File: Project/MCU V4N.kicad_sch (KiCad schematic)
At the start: 10 parts, among them U59 STM32F072CBT6

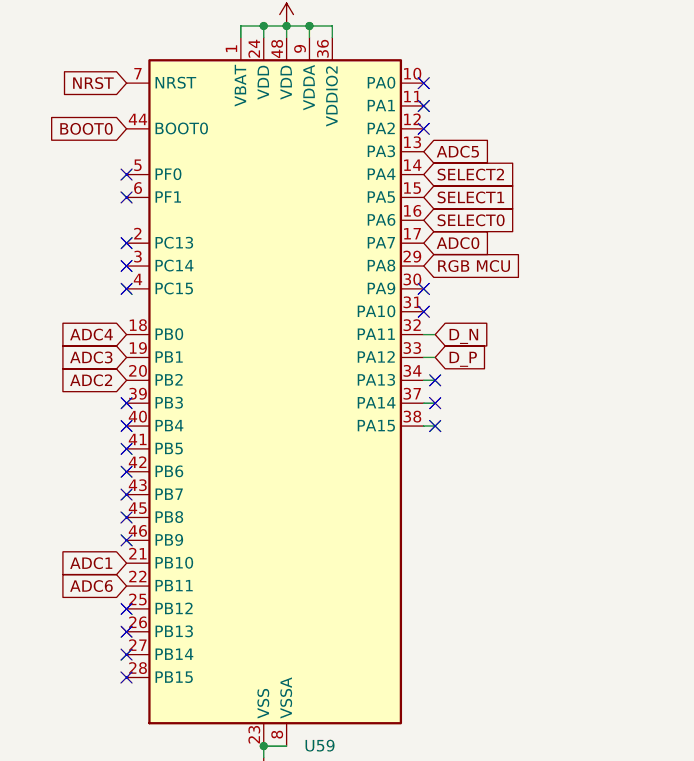
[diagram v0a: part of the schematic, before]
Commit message: pin revision
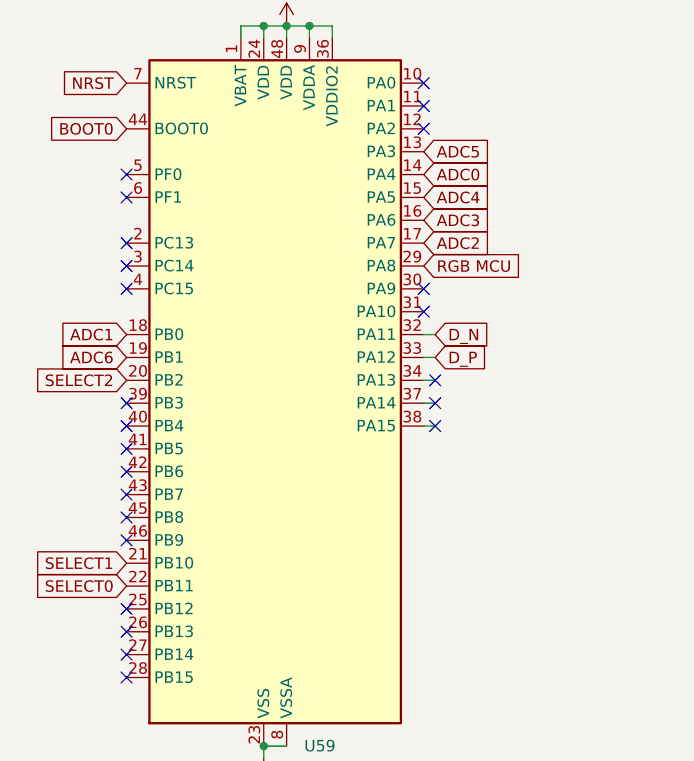
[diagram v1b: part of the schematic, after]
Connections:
- net ADC0: now also U59.14 (PA4); no longer U59.17 (PA7)
- net ADC1: now also U59.18 (PB0); no longer U59.21 (PB10)
- net ADC2: now also U59.17 (PA7); no longer U59.20 (PB2)
- net ADC3: now also U59.16 (PA6); no longer U59.19 (PB1)
- net ADC4: now also U59.15 (PA5); no longer U59.18 (PB0)
- net ADC6: now also U59.19 (PB1); no longer U59.22 (PB11)
- net SELECT0: now also U59.22 (PB11); no longer U59.16 (PA6)
- net SELECT1: now also U59.21 (PB10); no longer U59.15 (PA5)
- net SELECT2: now also U59.20 (PB2); no longer U59.14 (PA4)
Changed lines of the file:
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@@
   (no_connect (at 21.59 90.17))
   (no_connect (at 21.59 36.83))
+  (no_connect (at 54.61 24.13))
   (no_connect (at 21.59 34.29))
   (no_connect (at 21.59 44.45))
-  (no_connect (at 54.61 29.21))
   (no_connect (at 21.59 62.23))
   (no_connect (at 21.59 69.85))
   (no_connect (at 21.59 59.69))
+  (no_connect (at 54.61 29.21))
   (no_connect (at 54.61 46.99))
   (no_connect (at 21.59 67.31))
@@
   (no_connect (at 21.59 82.55))
   (no_connect (at 21.59 87.63))
+  (no_connect (at 54.61 26.67))
   (no_connect (at 55.88 59.69))
   (no_connect (at 21.59 46.99))
@@
   (no_connect (at 54.61 49.53))
   (no_connect (at 21.59 41.91))
-  (no_connect (at 54.61 24.13))
-  (no_connect (at 54.61 26.67))
   (wire (pts (xy 36.83 17.78) (xy 36.83 19.05))
     (stroke (width 0) (type default))
@@
     )
   )
-  (global_label "ADC3" (shape input) (at 21.59 54.61 180) (fields_autoplaced)
+  (global_label "ADC3" (shape input) (at 54.61 39.37 0) (fields_autoplaced)
+    (effects (font (size 1.27 1.27)) (justify left))
+    (property "Intersheetrefs" "${INTERSHEET_REFS}" (at 61.6997 39.37 0)
+      (effects (font (size 1.27 1.27)) (justify left) hide)
+    )
+  )
+  (global_label "ADC5" (shape input) (at 54.61 31.75 0) (fields_autoplaced)
+    (effects (font (size 1.27 1.27)) (justify left))
+    (property "Intersheetrefs" "${INTERSHEET_REFS}" (at 61.6997 31.75 0)
+      (effects (font (size 1.27 1.27)) (justify left) hide)
+    )
+  )
+  (global_label "ADC0" (shape input) (at 54.61 34.29 0) (fields_autoplaced)
+    (effects (font (size 1.27 1.27)) (justify left))
+    (property "Intersheetrefs" "${INTERSHEET_REFS}" (at 61.6997 34.29 0)
+      (effects (font (size 1.27 1.27)) (justify left) hide)
+    )
+  )
+  (global_label "ADC6" (shape input) (at 21.59 54.61 180) (fields_autoplaced)
     (effects (font (size 1.27 1.27)) (justify right))
     (property "Intersheetrefs" "${INTERSHEET_REFS}" (at 14.5003 54.61 0)
@@
     )
   )
-  (global_label "ADC5" (shape input) (at 54.61 31.75 0) (fields_autoplaced)
-    (effects (font (size 1.27 1.27)) (justify left))
-    (property "Intersheetrefs" "${INTERSHEET_REFS}" (at 61.6997 31.75 0)
-      (effects (font (size 1.27 1.27)) (justify left) hide)
-    )
-  )
-  (global_label "ADC0" (shape input) (at 54.61 41.91 0) (fields_autoplaced)
+  (global_label "D_P" (shape input) (at 55.88 54.61 0) (fields_autoplaced)
+    (effects (font (size 1.27 1.27)) (justify left))
+    (property "Intersheetrefs" "${INTERSHEET_REFS}" (at 62.2934 54.61 0)
+      (effects (font (size 1.27 1.27)) (justify left) hide)
+    )
+  )
+  (global_label "ADC2" (shape input) (at 54.61 41.91 0) (fields_autoplaced)
     (effects (font (size 1.27 1.27)) (justify left))
     (property "Intersheetrefs" "${INTERSHEET_REFS}" (at 61.6997 41.91 0)
@@
     )
   )
-  (global_label "ADC6" (shape input) (at 21.59 80.01 180) (fields_autoplaced)
-    (effects (font (size 1.27 1.27)) (justify right))
-    (property "Intersheetrefs" "${INTERSHEET_REFS}" (at 14.5003 80.01 0)
-      (effects (font (size 1.27 1.27)) (justify right) hide)
-    )
-  )
-  (global_label "D_P" (shape input) (at 55.88 54.61 0) (fields_autoplaced)
-    (effects (font (size 1.27 1.27)) (justify left))
-    (property "Intersheetrefs" "${INTERSHEET_REFS}" (at 62.2934 54.61 0)
-      (effects (font (size 1.27 1.27)) (justify left) hide)
-    )
-  )
-  (global_label "ADC2" (shape input) (at 21.59 57.15 180) (fields_autoplaced)
-    (effects (font (size 1.27 1.27)) (justify right))
-    (property "Intersheetrefs" "${INTERSHEET_REFS}" (at 14.5003 57.15 0)
-      (effects (font (size 1.27 1.27)) (justify right) hide)
-    )
-  )
-  (global_label "SELECT1" (shape input) (at 54.61 36.83 0) (fields_autoplaced)
-    (effects (font (size 1.27 1.27)) (justify left))
-    (property "Intersheetrefs" "${INTERSHEET_REFS}" (at 64.8443 36.83 0)
-      (effects (font (size 1.27 1.27)) (justify left) hide)
+  (global_label "SELECT1" (shape input) (at 21.59 77.47 180) (fields_autoplaced)
+    (effects (font (size 1.27 1.27)) (justify right))
+    (property "Intersheetrefs" "${INTERSHEET_REFS}" (at 11.3557 77.47 0)
+      (effects (font (size 1.27 1.27)) (justify right) hide)
     )
   )
@@
     )
   )
-  (global_label "SELECT2" (shape input) (at 54.61 34.29 0) (fields_autoplaced)
-    (effects (font (size 1.27 1.27)) (justify left))
-    (property "Intersheetrefs" "${INTERSHEET_REFS}" (at 64.8443 34.29 0)
-      (effects (font (size 1.27 1.27)) (justify left) hide)
-    )
-  )
-  (global_label "SELECT0" (shape input) (at 54.61 39.37 0) (fields_autoplaced)
-    (effects (font (size 1.27 1.27)) (justify left))
-    (property "Intersheetrefs" "${INTERSHEET_REFS}" (at 64.8443 39.37 0)
-      (effects (font (size 1.27 1.27)) (justify left) hide)
-    )
-  )
-  (global_label "ADC4" (shape input) (at 21.59 52.07 180) (fields_autoplaced)
+  (global_label "SELECT2" (shape input) (at 21.59 57.15 180) (fields_autoplaced)
+    (effects (font (size 1.27 1.27)) (justify right))
+    (property "Intersheetrefs" "${INTERSHEET_REFS}" (at 11.3557 57.15 0)
+      (effects (font (size 1.27 1.27)) (justify right) hide)
+    )
+  )
+  (global_label "SELECT0" (shape input) (at 21.59 80.01 180) (fields_autoplaced)
+    (effects (font (size 1.27 1.27)) (justify right))
+    (property "Intersheetrefs" "${INTERSHEET_REFS}" (at 11.3557 80.01 0)
+      (effects (font (size 1.27 1.27)) (justify right) hide)
+    )
+  )
+  (global_label "ADC4" (shape input) (at 54.61 36.83 0) (fields_autoplaced)
+    (effects (font (size 1.27 1.27)) (justify left))
+    (property "Intersheetrefs" "${INTERSHEET_REFS}" (at 61.6997 36.83 0)
+      (effects (font (size 1.27 1.27)) (justify left) hide)
+    )
+  )
+  (global_label "NRST" (shape input) (at 105.41 81.915 180) (fields_autoplaced)
+    (effects (font (size 1.27 1.27)) (justify right))
+    (property "Intersheetrefs" "${INTERSHEET_REFS}" (at 97.7266 81.915 0)
+      (effects (font (size 1.27 1.27)) (justify right) hide)
+    )
+  )
+  (global_label "BOOT0" (shape input) (at 106.68 65.405 0) (fields_autoplaced)
+    (effects (font (size 1.27 1.27)) (justify left))
+    (property "Intersheetrefs" "${INTERSHEET_REFS}" (at 115.2012 65.3256 0)
+      (effects (font (size 1.27 1.27)) (justify left) hide)
+    )
+  )
+  (global_label "ADC1" (shape input) (at 21.59 52.07 180) (fields_autoplaced)
     (effects (font (size 1.27 1.27)) (justify right))
     (property "Intersheetrefs" "${INTERSHEET_REFS}" (at 14.5003 52.07 0)
       (effects (font (size 1.27 1.27)) (justify right) hide)
     )
-  )
-  (global_label "NRST" (shape input) (at 105.41 81.915 180) (fields_autoplaced)
-    (effects (font (size 1.27 1.27)) (justify right))
-    (property "Intersheetrefs" "${INTERSHEET_REFS}" (at 97.7266 81.915 0)
-      (effects (font (size 1.27 1.27)) (justify right) hide)
-    )
-  )
-  (global_label "BOOT0" (shape input) (at 106.68 65.405 0) (fields_autoplaced)
-    (effects (font (size 1.27 1.27)) (justify left))
-    (property "Intersheetrefs" "${INTERSHEET_REFS}" (at 115.2012 65.3256 0)
-      (effects (font (size 1.27 1.27)) (justify left) hide)
-    )
-  )
-  (global_label "ADC1" (shape input) (at 21.59 77.47 180) (fields_autoplaced)
-    (effects (font (size 1.27 1.27)) (justify right))
-    (property "Intersheetrefs" "${INTERSHEET_REFS}" (at 13.7667 77.47 0)
-      (effects (font (size 1.27 1.27)) (justify right) hide)
-    )

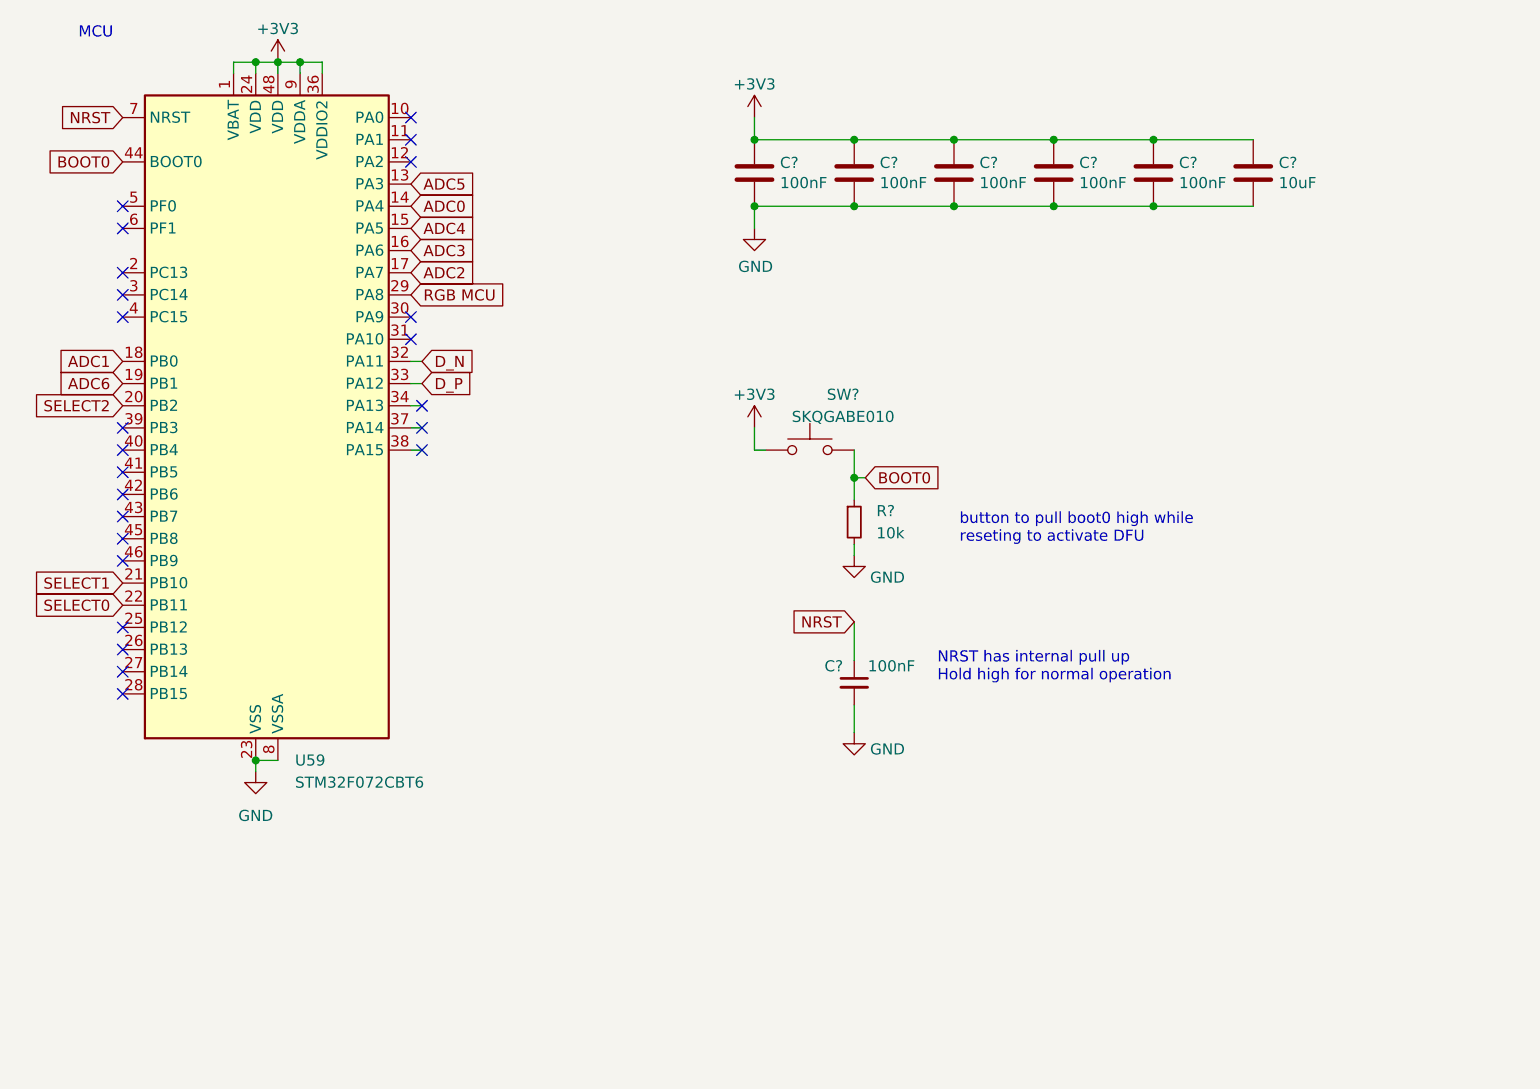
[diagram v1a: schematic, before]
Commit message: update
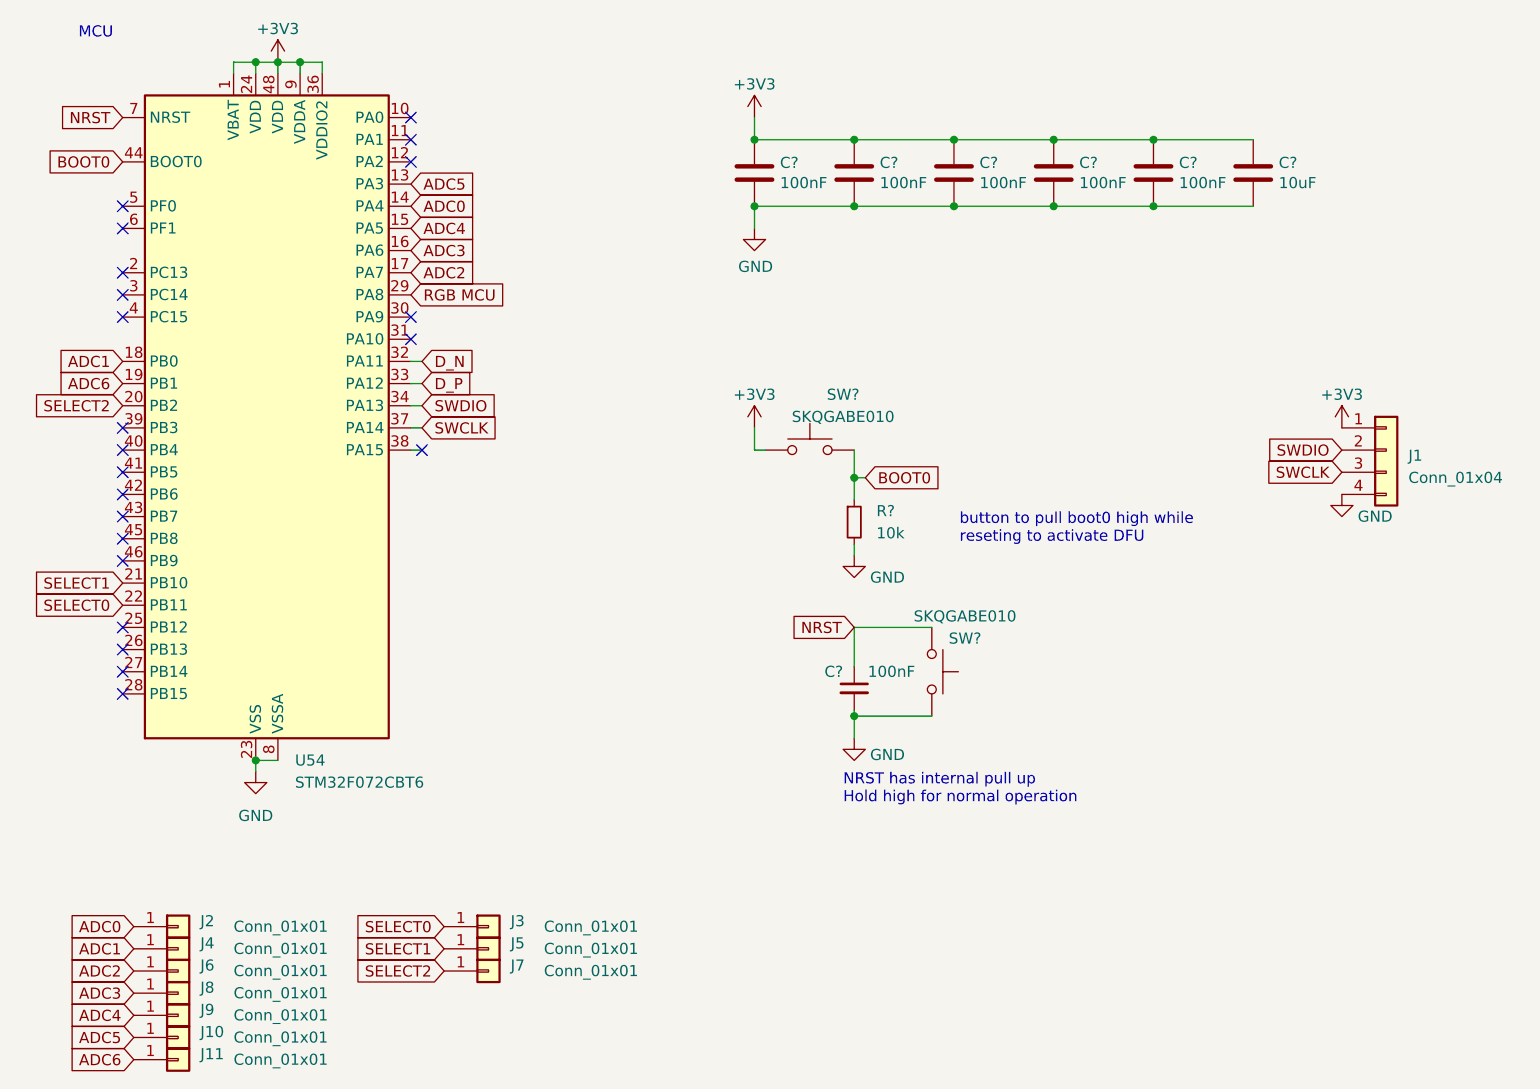
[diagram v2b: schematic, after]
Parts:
- added J1: Conn_01x04, Connector_PinHeader_2.54mm:PinHeader_1x04_P2.54mm_Vertical, symbol Connector_Generic:Conn_01x04
- added J10, J11, J2, J3, J4, J5, J6, J7, J8, J9: Conn_01x01, TestPoint:TestPoint_THTPad_D1.5mm_Drill0.7mm, symbol Connector_Generic:Conn_01x01
- added SW?: SKQGABE010, Button_Switch_SMD:SW_SPST_SKQG_WithoutStem, symbol Switch:SW_Push
- renumbered U59 to U54
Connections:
- net +3V3: now also J1.1 (Pin_1)
- net ADC0: now also J2.1 (Pin_1)
- net ADC1: now also J4.1 (Pin_1)
- net ADC2: now also J6.1 (Pin_1)
- net ADC3: now also J8.1 (Pin_1)
- net ADC4: now also J9.1 (Pin_1)
- net ADC5: now also J10.1 (Pin_1)
- net ADC6: now also J11.1 (Pin_1)
- net GND: now also J1.4 (Pin_4), SW?.2
- net NRST: now also SW?.1
- net SELECT0: now also J3.1 (Pin_1)
- net SELECT1: now also J5.1 (Pin_1)
- net SELECT2: now also J7.1 (Pin_1)
- net SWDIO: now reaches U54.34 (PA13)
- net SWDIO: now also J1.2 (Pin_2)
- net SWCLK: now reaches U54.37 (PA14)
- net SWCLK: now also J1.3 (Pin_3)
- no-connect marks 24 -> 22
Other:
- moved on the sheet: C?
